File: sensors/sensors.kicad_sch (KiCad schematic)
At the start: 6 parts, among them J1 Conn 1x3, U1 TCRT5000

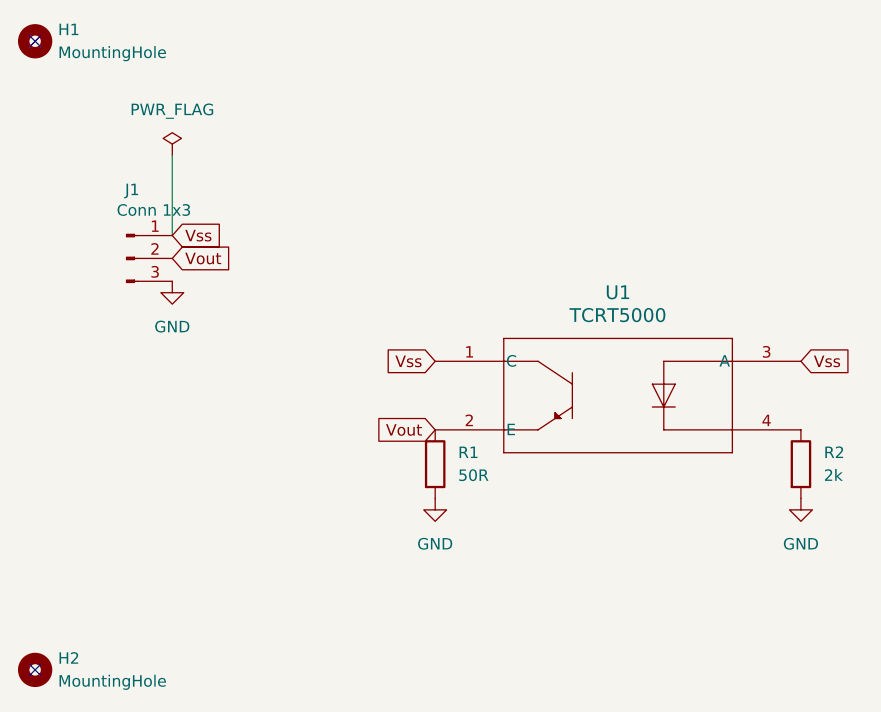
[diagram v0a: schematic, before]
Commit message: Changed the layout of the files
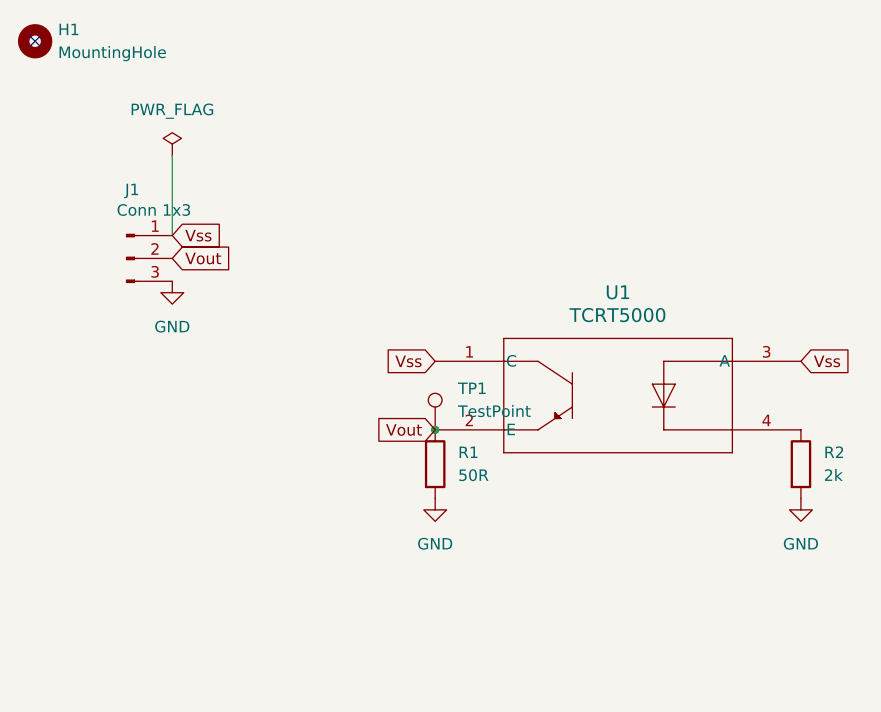
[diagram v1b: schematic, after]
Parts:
- removed H2: MountingHole, MountingHole:MountingHole_3.2mm_M3, symbol Mechanical:MountingHole
- added TP1: TestPoint, TestPoint:TestPoint_Plated_Hole_D2.0mm, symbol Connector:TestPoint
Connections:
- net Vout: now also TP1.1
- no-connect marks 2 -> 1
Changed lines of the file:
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@@
 	(generator_version "9.0")
 	(paper "A4")
+	(junction
+		(at 95.25 87.63)
+		(diameter 0)
+		(color 0 0 0 0)
+	)
 	(no_connect
 		(at 50.8 44.45)
-	)
-	(no_connect
-		(at 50.8 114.3)
 	)
 	(wire
@@
 	)
 	(symbol
-		(lib_id "Mechanical:MountingHole")
-		(at 50.8 114.3 0)
-		(unit 1)
-		(exclude_from_sim no)
-		(in_bom no)
-		(on_board yes)
-		(dnp no)
-		(fields_autoplaced yes)
-		(property "Reference" "H2"
-			(at 53.34 113.0299 0)
-			(effects
-				(font
-					(size 1.27 1.27)
-				)
-				(justify left)
-			)
-		)
-		(property "Value" "MountingHole"
-			(at 53.34 115.5699 0)
-			(effects
-				(font
-					(size 1.27 1.27)
-				)
-				(justify left)
-			)
-		)
-		(property "Footprint" "MountingHole:MountingHole_3.2mm_M3"
-			(at 50.8 114.3 0)
-			(effects
-				(font
-					(size 1.27 1.27)
-				)
-				(hide yes)
-			)
-		)
-		(property "Datasheet" "~"
-			(at 50.8 114.3 0)
-			(effects
-				(font
-					(size 1.27 1.27)
-				)
-				(hide yes)
-			)
-		)
-		(property "Description" "Mounting Hole without connection"
-			(at 50.8 114.3 0)
-			(effects
-				(font
-					(size 1.27 1.27)
-				)
-				(hide yes)
-			)
-		)
-		(instances
-			(project ""
-				(path "/7a5c889d-d948-4110-bf7e-4c334aa2755f"
-					(reference "H2")
-					(unit 1)
-				)
-			)
-		)
-	)
-	(symbol
 		(lib_id "lib:TCRT5000")
 		(at 95.25 80.01 0)
@@
 					(unit 1)
 				)
+			)
+		)
+	)
+	(symbol
+		(lib_id "Connector:TestPoint")
+		(at 95.25 87.63 0)
+		(unit 1)
+		(exclude_from_sim no)
+		(in_bom yes)
+		(on_board yes)
+		(dnp no)
+		(fields_autoplaced yes)
+		(property "Reference" "TP1"
+			(at 97.79 83.0579 0)
+			(effects
+				(font
+					(size 1.27 1.27)
+				)
+				(justify left)
+			)
+		)
+		(property "Value" "TestPoint"
+			(at 97.79 85.5979 0)
+			(effects
+				(font
+					(size 1.27 1.27)
+				)
+				(justify left)
+			)
+		)
+		(property "Footprint" "TestPoint:TestPoint_Plated_Hole_D2.0mm"
+			(at 100.33 87.63 0)
+			(effects
+				(font
+					(size 1.27 1.27)
+				)
+				(hide yes)
+			)
+		)
+		(property "Datasheet" "~"
+			(at 100.33 87.63 0)
+			(effects
+				(font
+					(size 1.27 1.27)
+				)
+				(hide yes)
+			)
+		)
+		(property "Description" "test point"
+			(at 95.25 87.63 0)
+			(effects
+				(font
+					(size 1.27 1.27)
+				)
+				(hide yes)
+			)
+		)
+		(pin "1"
+		)
+		(instances
+			(project ""
+				(path "/7a5c889d-d948-4110-bf7e-4c334aa2755f"
+					(reference "TP1")
+					(unit 1)
+				)
